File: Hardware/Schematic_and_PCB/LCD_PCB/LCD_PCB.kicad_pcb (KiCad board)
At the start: 2 copper layers, 97 x 64.8 mm, 10 parts, among them J1 LCD_display, J2 Conn_01x10, SW1 Button_down, SW2 Button_up, SW3 Button_ok, SW4 Button_back, SW5 SW_Push

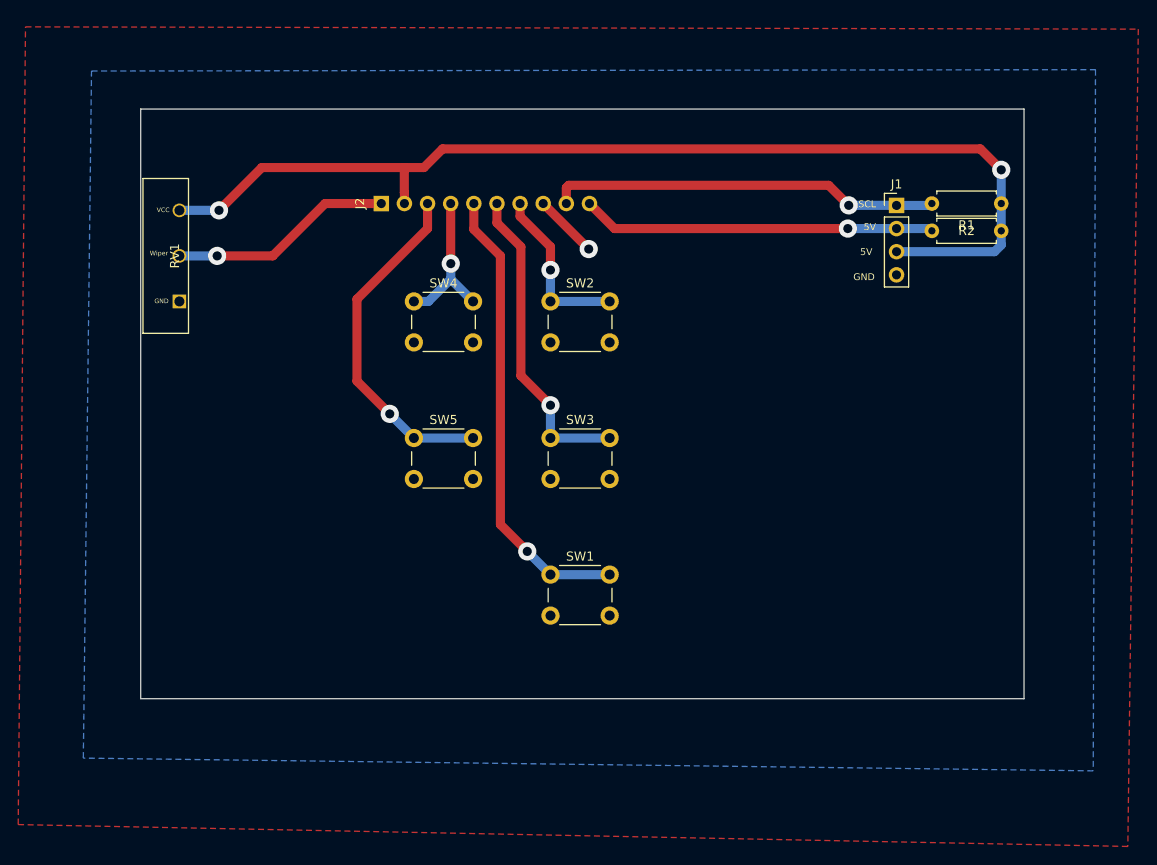
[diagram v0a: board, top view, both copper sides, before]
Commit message: Finalize LCD PCB
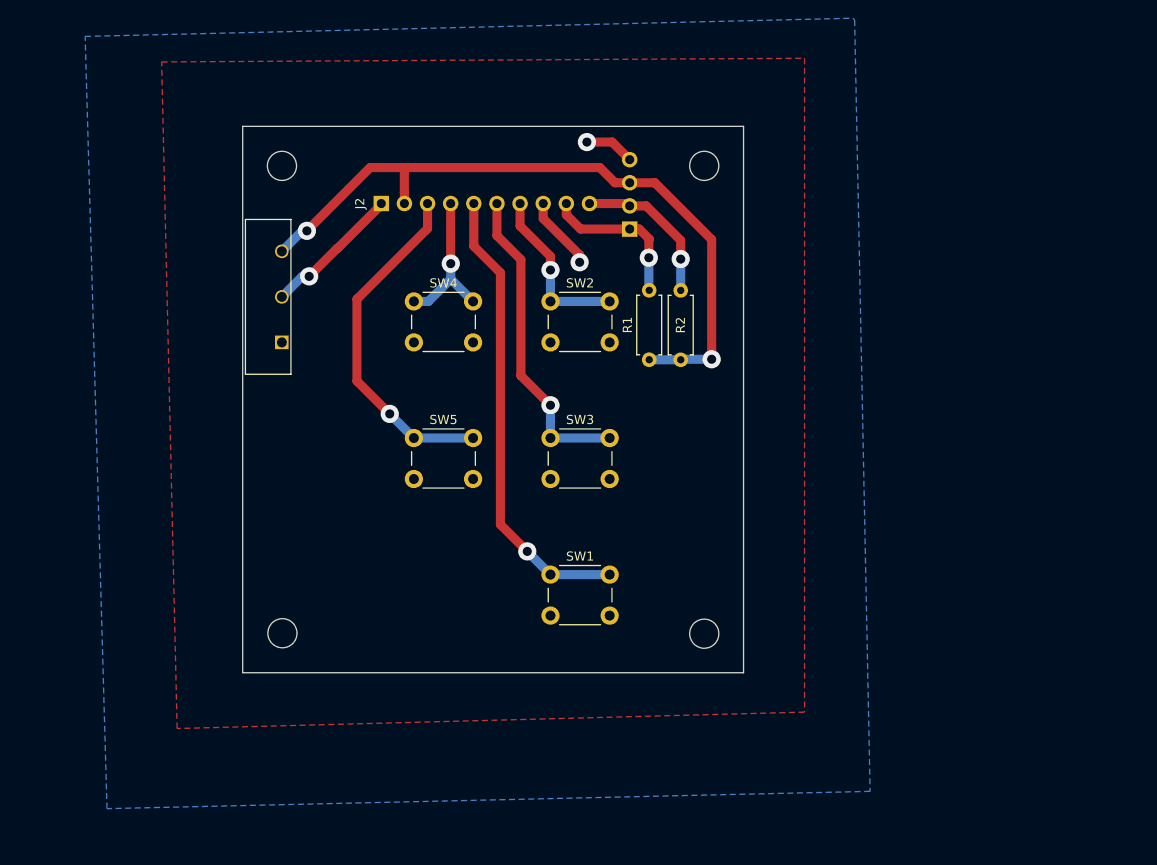
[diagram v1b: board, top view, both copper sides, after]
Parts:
- added H1: MountingHole, MountingHole:MountingHole_3.2mm_M3, F.Cu at (94.0, 36.6)
- added H2: MountingHole, MountingHole:MountingHole_3.2mm_M3, F.Cu at (140.4, 36.6)
- added H3: MountingHole, MountingHole:MountingHole_3.2mm_M3, F.Cu at (94.1, 87.9)
- added H4: MountingHole, MountingHole:MountingHole_3.2mm_M3, F.Cu at (140.4, 88.0)
- J1: moved to B.Cu
- moved R1 42.3 mm to (134.3, 57.9), turned to 90 degrees
- moved R2 37.9 mm to (137.8, 57.9), turned to 90 degrees
- moved J1 29.4 mm to (132.2, 43.5)
- moved RV1 12.1 mm to (94.0, 51.0)
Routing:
- net 5V: track 118.0 -> 78.4 mm
- net lcd SCL: track 43.3 -> 17.2 mm
- net lcd SDA: track 39.2 -> 17.2 mm
- net control panel pot: track 24.6 -> 15.2 mm
- net GND: track 7.07 -> 13.6 mm, vias 1 -> 2
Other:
- board size 97 x 64.8 mm -> 55 x 60 mm
- board text removed: "5V"
- board text removed: "GND"
- board text removed: "SCL"
